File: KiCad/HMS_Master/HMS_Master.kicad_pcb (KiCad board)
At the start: 2 copper layers, 150 x 90 mm, 28 parts, among them Q1 S8050, U1 ESP32-DEVKITC-32UE, U11 MICROSD_SPI_3V3, U14 GAS_FLOW_SENSOR_SOCKET, U15 GAS_RETURN_SENSOR_SOCKET, U16 WOOD_FLOW_SENSOR_SOCKET, U17 WOOD_RETURN_SENSOR_SOCKET, U18 WOOD_BOILER_SENSOR_SOCKET, U19 BUZZER_SOCKET, U20 BOILER_ROOM_SENSOR_SOCKET, U21 GAS_AC_PRESENT_SOCKET, U22 WOOD_AC_PRESENT_SOCKET, U23 DISPLAY_POWER_SOCKET, U24 DISPLAY_SPI_SOCKET, U25 DISPLAY_CONTOL_SOCKET, U26 USB_Micro-B_Socket, U3 MAX6675, U9 DS3231+AT24C32

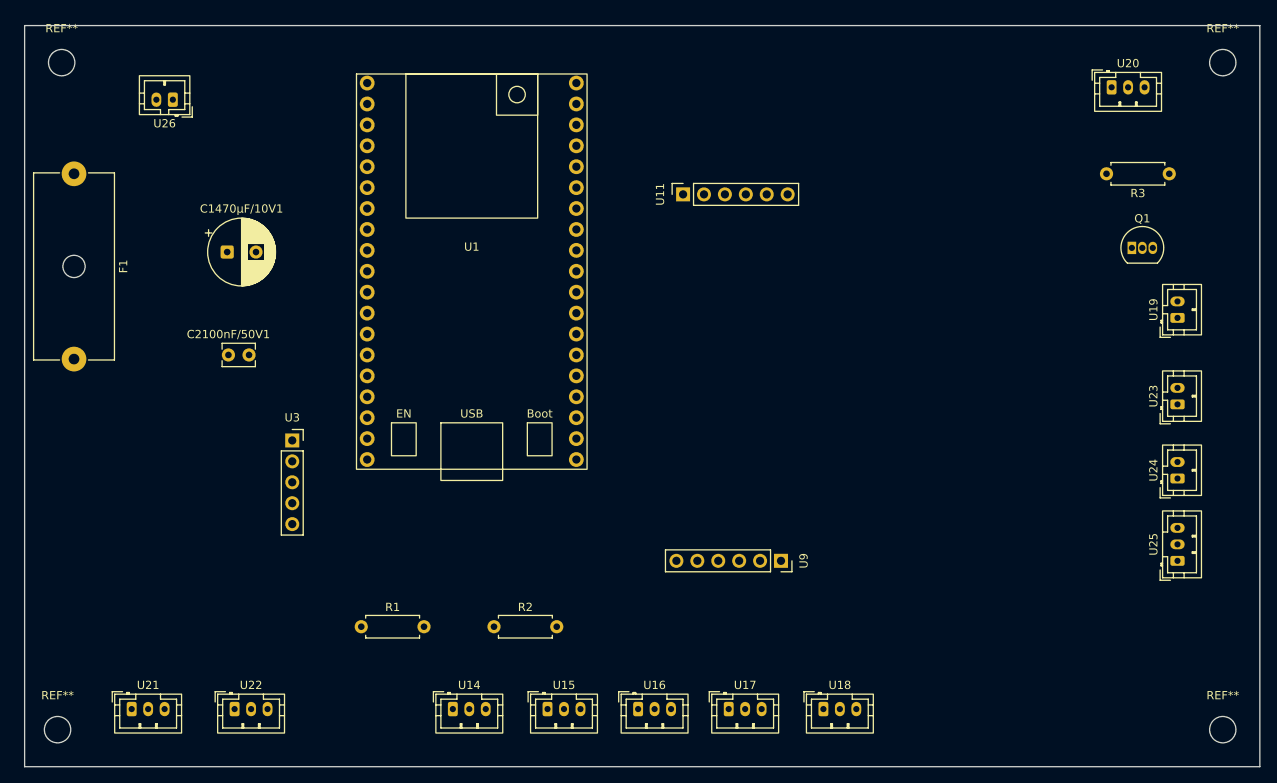
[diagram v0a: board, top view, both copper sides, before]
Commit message: Finished PCB
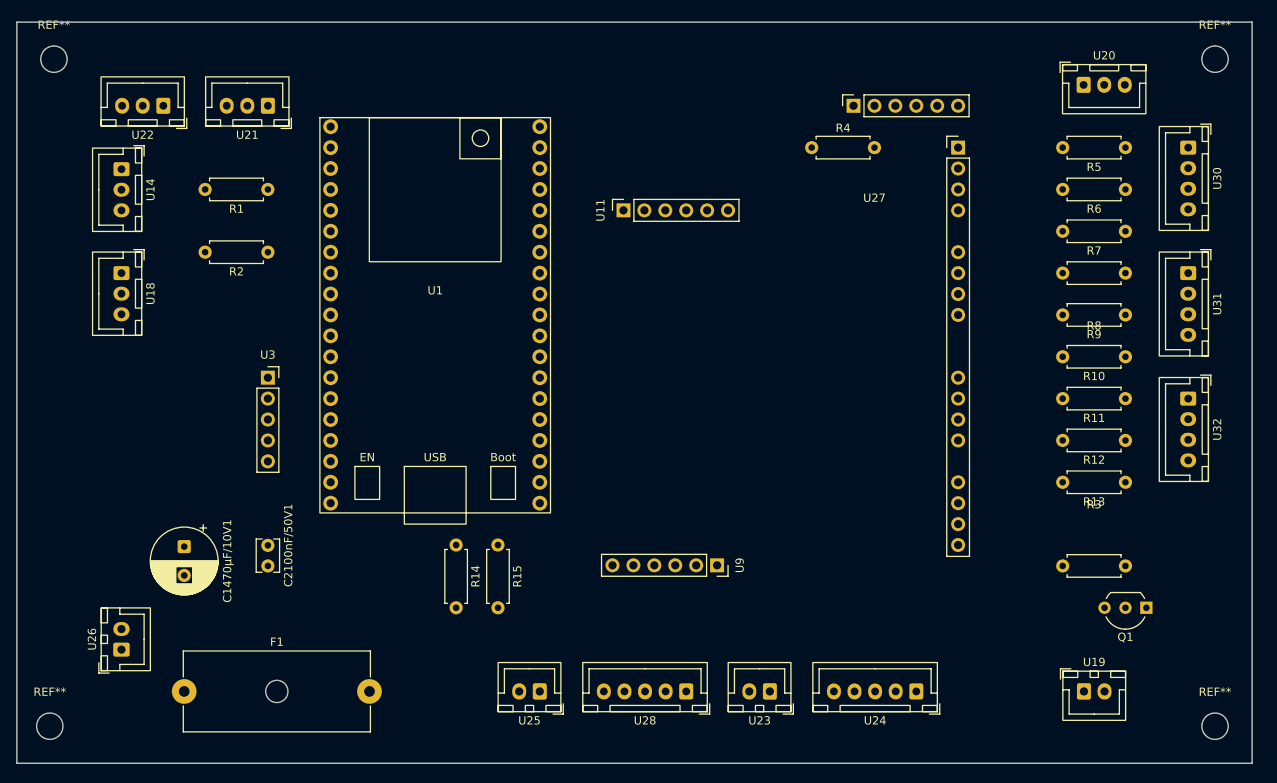
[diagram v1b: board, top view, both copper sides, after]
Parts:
- removed U15: GAS_RETURN_SENSOR_SOCKET, Connector_JST:JST_PH_B3B-PH-K_1x03_P2.00mm_Vertical
- removed U16: WOOD_FLOW_SENSOR_SOCKET, Connector_JST:JST_PH_B3B-PH-K_1x03_P2.00mm_Vertical
- removed U17: WOOD_RETURN_SENSOR_SOCKET, Connector_JST:JST_PH_B3B-PH-K_1x03_P2.00mm_Vertical
- added R10: 220Ω, Resistor_THT:R_Axial_DIN0207_L6.3mm_D2.5mm_P7.62mm_Horizontal, F.Cu at (233.7, 109.2)
- added R11: 220Ω, Resistor_THT:R_Axial_DIN0207_L6.3mm_D2.5mm_P7.62mm_Horizontal, F.Cu at (233.7, 114.3)
- added R12: 220Ω, Resistor_THT:R_Axial_DIN0207_L6.3mm_D2.5mm_P7.62mm_Horizontal, F.Cu at (233.7, 119.4)
- added R13: 220Ω, Resistor_THT:R_Axial_DIN0207_L6.3mm_D2.5mm_P7.62mm_Horizontal, F.Cu at (233.7, 124.5)
- added R14: 100Ω, Resistor_THT:R_Axial_DIN0207_L6.3mm_D2.5mm_P7.62mm_Horizontal, F.Cu at (152.4, 132.1)
- added R15: 100Ω, Resistor_THT:R_Axial_DIN0207_L6.3mm_D2.5mm_P7.62mm_Horizontal, F.Cu at (157.5, 132.1)
- added R4: 10kΩ, Resistor_THT:R_Axial_DIN0207_L6.3mm_D2.5mm_P7.62mm_Horizontal, F.Cu at (195.6, 83.8)
- added R5: 220Ω, Resistor_THT:R_Axial_DIN0207_L6.3mm_D2.5mm_P7.62mm_Horizontal, F.Cu at (233.7, 83.8)
- added R6: 220Ω, Resistor_THT:R_Axial_DIN0207_L6.3mm_D2.5mm_P7.62mm_Horizontal, F.Cu at (233.7, 88.9)
- added R7: 220Ω, Resistor_THT:R_Axial_DIN0207_L6.3mm_D2.5mm_P7.62mm_Horizontal, F.Cu at (233.7, 94.0)
- added R8: 220Ω, Resistor_THT:R_Axial_DIN0207_L6.3mm_D2.5mm_P7.62mm_Horizontal, F.Cu at (233.7, 99.1)
- added R9: 220Ω, Resistor_THT:R_Axial_DIN0207_L6.3mm_D2.5mm_P7.62mm_Horizontal, F.Cu at (233.7, 104.1)
- added U27: SERVO16-1A-SLD, HMS_Footprints:SERVO16-1A-SLD, F.Cu at (205.7, 86.4)
- added U28: DISPLAY2_DATA_SOCKET, Connector_JST:JST_XH_B5B-XH-A_1x05_P2.50mm_Vertical, F.Cu at (180.3, 149.9)
- added U30: LED_GAS_SOCKET, Connector_JST:JST_XH_B4B-XH-A_1x04_P2.50mm_Vertical, F.Cu at (241.3, 83.8)
- added U31: LED_WOOD_SOCKET, Connector_JST:JST_XH_B4B-XH-A_1x04_P2.50mm_Vertical, F.Cu at (241.3, 99.1)
- added U32: LED_STATUS_SOCKET, Connector_JST:JST_XH_B4B-XH-A_1x04_P2.50mm_Vertical, F.Cu at (241.3, 114.3)
- Q1: footprint Package_TO_SOT_THT:TO-92_Inline -> Package_TO_SOT_THT:TO-92_Inline_Wide
- R2: value 33Ω_NDP -> 33Ω
- U14: value GAS_FLOW_SENSOR_SOCKET -> PIPE_SENSORS_SOCKET; footprint Connector_JST:JST_PH_B3B-PH-K_1x03_P2.00mm_Vertical -> Connector_JST:JST_XH_B3B-XH-A_1x03_P2.50mm_Vertical
- U18, U20, U21, U22: footprint Connector_JST:JST_PH_B3B-PH-K_1x03_P2.00mm_Vertical -> Connector_JST:JST_XH_B3B-XH-A_1x03_P2.50mm_Vertical
- U19, U26: footprint Connector_JST:JST_PH_B2B-PH-K_1x02_P2.00mm_Vertical -> Connector_JST:JST_XH_B2B-XH-A_1x02_P2.50mm_Vertical
- U23: value DISPLAY_POWER_SOCKET -> DISPLAY1_POWER_SOCKET; footprint Connector_JST:JST_PH_B2B-PH-K_1x02_P2.00mm_Vertical -> Connector_JST:JST_XH_B2B-XH-A_1x02_P2.50mm_Vertical
- U24: value DISPLAY_SPI_SOCKET -> DISPLAY1_DATA_SOCKET; footprint Connector_JST:JST_PH_B2B-PH-K_1x02_P2.00mm_Vertical -> Connector_JST:JST_XH_B5B-XH-A_1x05_P2.50mm_Vertical
- U25: value DISPLAY_CONTOL_SOCKET -> DISPLAY2_POWER_SOCKET; footprint Connector_JST:JST_PH_B3B-PH-K_1x03_P2.00mm_Vertical -> Connector_JST:JST_XH_B2B-XH-A_1x02_P2.50mm_Vertical
- moved U18 100.3 mm to (111.8, 99.1), turned to -90 degrees
- moved U25 79.0 mm to (162.6, 149.9), turned to 180 degrees
- moved U14 76.9 mm to (111.8, 86.4), turned to -90 degrees
- moved U21 75.1 mm to (129.5, 78.7), turned to 180 degrees
- moved U22 73.8 mm to (116.8, 78.7), turned to 180 degrees
- moved U26 67.1 mm to (111.8, 144.8), turned to 90 degrees
- moved F1 64.3 mm to (119.4, 149.9), turned to 0 degrees
- moved U23 60.5 mm to (190.5, 149.9), turned to 180 degrees
- moved R1 54.3 mm to (129.5, 88.9), turned to 180 degrees
- moved R2 53.1 mm to (129.5, 96.5), turned to 180 degrees
- moved R3 49.3 mm to (226.1, 134.6), turned to 0 degrees
- moved U19 46.8 mm to (228.6, 149.9), turned to 0 degrees
- moved Q1 43.7 mm to (236.2, 139.7), turned to 180 degrees
- moved U24 40.9 mm to (208.3, 149.9), turned to 180 degrees
- moved C1470µF/10V1 36.2 mm to (119.4, 132.3), turned to -90 degrees
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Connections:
- U1 pad 12: /01_ESP32/WOOD_AC_PRESENT -> /01_ESP32/CHIMNEY_TEMPERATURE_CS
- U1 pad 15: unconnected-(U1-GPIO13-Pad15) -> /01_ESP32/MICROSD_CS
- U1 pad 29: /01_ESP32/DISPLAY_CS -> /01_ESP32/DISPLAY1_CS
- U1 pad 32: /01_ESP32/CHIMNEY_TEMPERATURE_CS -> /01_ESP32/DISPLAY2_CS
- U1 pad 8: /01_ESP32/MICROSD_CS -> /01_ESP32/WOOD_AC_PRESENT
- U25 pad 1: /01_ESP32/DISPLAY_RESET -> /01_ESP32/PWR_GND
- U25 pad 2: /01_ESP32/DISPLAY_DC -> /01_ESP32/PWR_3V3_OUT
